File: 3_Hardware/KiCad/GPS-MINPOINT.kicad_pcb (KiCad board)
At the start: 2 copper layers, 2 parts, among them J1 110990030, U2 PIC24FJ64GA002-I/SP

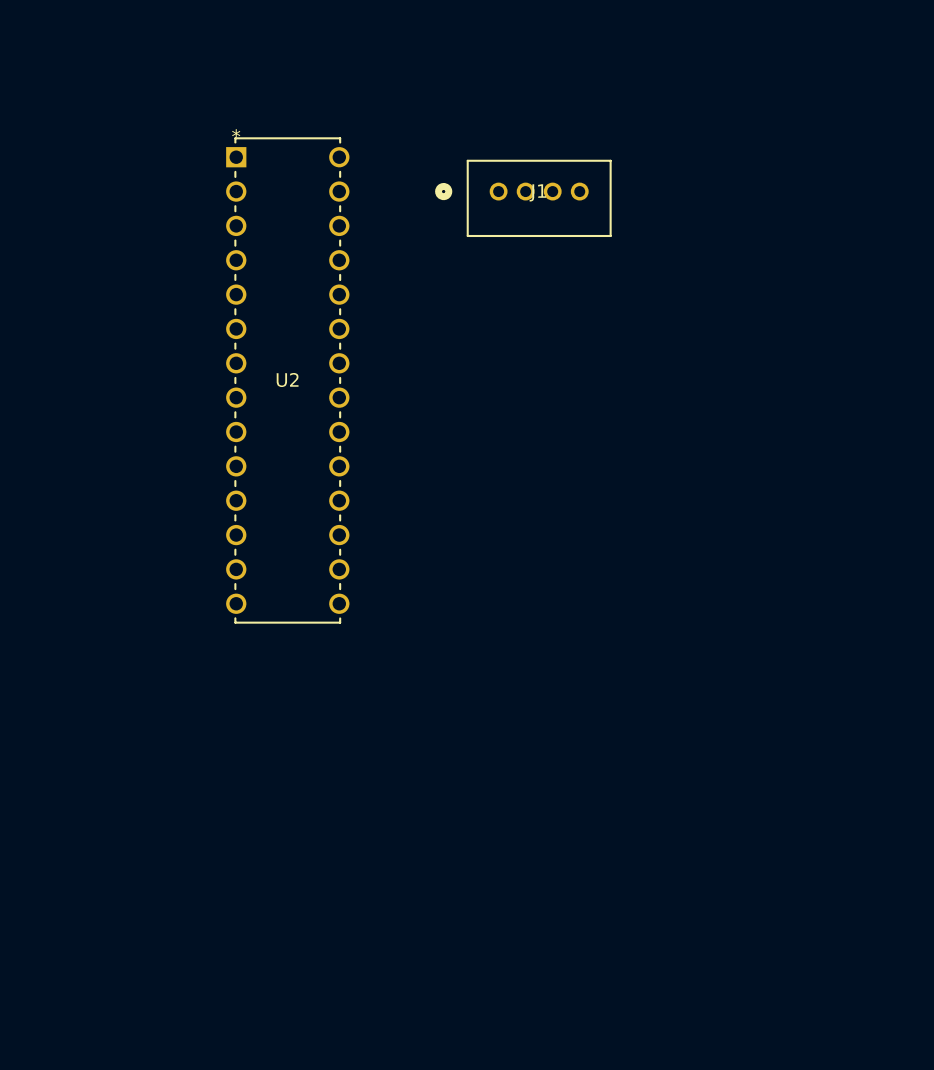
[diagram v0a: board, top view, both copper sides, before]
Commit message: Upload of finished PCB design
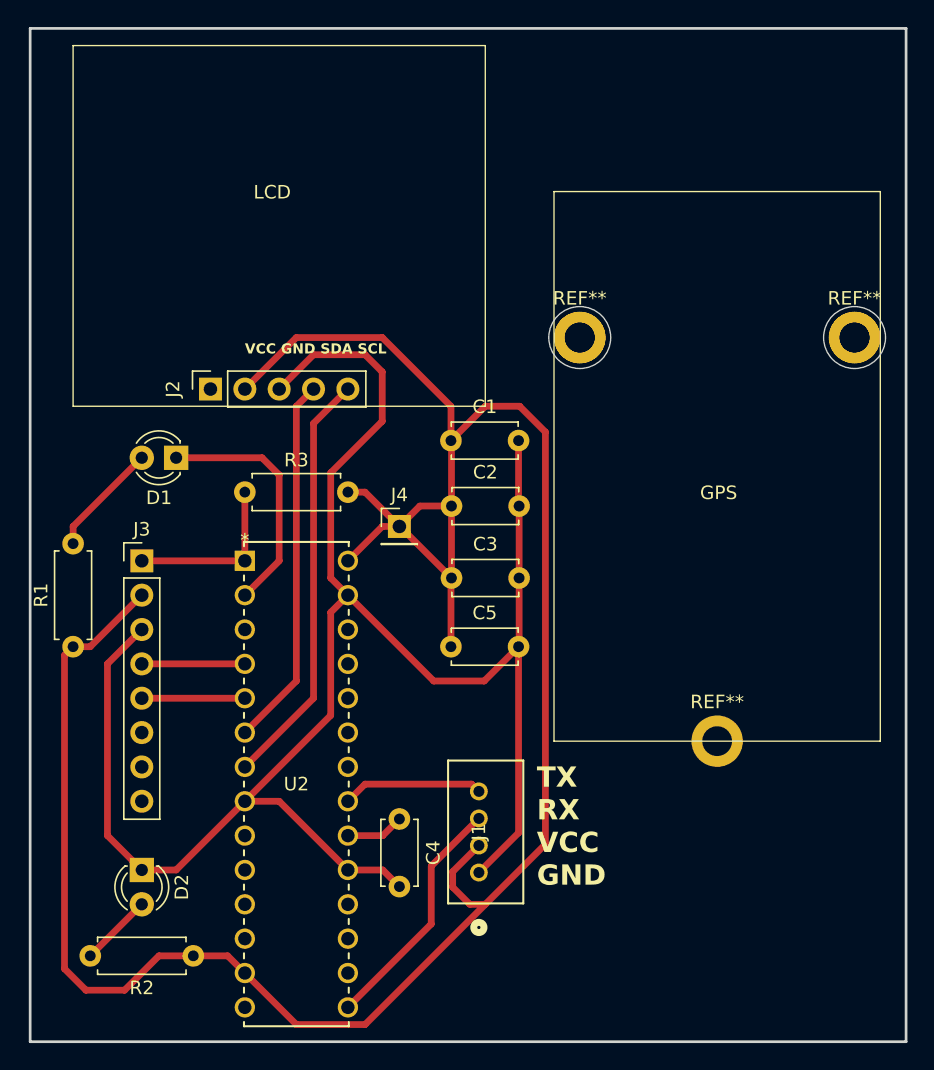
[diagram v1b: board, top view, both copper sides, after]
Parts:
- added ?: , , F.Cu at (167.6, 81.9)
- added ?: , , F.Cu at (188.0, 81.9)
- added C1: 10uF, Capacitor_THT:C_Disc_D4.7mm_W2.5mm_P5.00mm, F.Cu at (158.1, 89.5)
- added C2: 100nF, Capacitor_THT:C_Disc_D4.7mm_W2.5mm_P5.00mm, F.Cu at (158.2, 94.4)
- added C3: 100nF, Capacitor_THT:C_Disc_D4.7mm_W2.5mm_P5.00mm, F.Cu at (158.2, 99.7)
- added C4: 10uF, Capacitor_THT:C_Disc_D4.7mm_W2.5mm_P5.00mm, F.Cu at (154.3, 117.5)
- added C5: 10uF, Capacitor_THT:C_Disc_D4.7mm_W2.5mm_P5.00mm, F.Cu at (158.1, 104.8)
- added D1: G_LED, LED_THT:LED_D3.0mm, F.Cu at (137.8, 90.8)
- added D2: R_LED, LED_THT:LED_D3.0mm, F.Cu at (135.3, 121.3)
- added J2: LCD, Connector_PinSocket_2.54mm:PinSocket_1x05_P2.54mm_Vertical, F.Cu at (140.3, 85.7)
- added J3: ProgrammerConnector, Connector_PinHeader_2.54mm:PinHeader_1x08_P2.54mm_Vertical, F.Cu at (135.3, 98.4)
- added J4: PWR, Connector_PinHeader_2.54mm:PinHeader_1x01_P2.54mm_Vertical, F.Cu at (154.3, 95.9)
- added R1: 220, Resistor_THT:R_Axial_DIN0207_L6.3mm_D2.5mm_P7.62mm_Horizontal, F.Cu at (130.2, 104.8)
- added R2: 220, Resistor_THT:R_Axial_DIN0207_L6.3mm_D2.5mm_P7.62mm_Horizontal, F.Cu at (139.1, 127.6)
- added R3: 10k, Resistor_THT:R_Axial_DIN0207_L6.3mm_D2.5mm_P7.62mm_Horizontal, F.Cu at (142.9, 93.3)
- added REF**: MountingHole_2.2mm_M2_DIN965_Pad, MountingHole:MountingHole_2.2mm_M2_DIN965_Pad, F.Cu at (167.6, 81.9)
- added REF**: MountingHole_2.2mm_M2_DIN965_Pad, MountingHole:MountingHole_2.2mm_M2_DIN965_Pad, F.Cu at (188.0, 81.9)
- added REF**: MountingHole_2.2mm_M2_DIN965_Pad, MountingHole:MountingHole_2.2mm_M2_DIN965_Pad, F.Cu at (177.8, 111.8)
- moved J1 50.4 mm to (160.2, 121.5), turned to 90 degrees
- moved U2 29.9 mm to (142.9, 98.4)
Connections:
- J1 pad 1: Net-(J1-Pad1) -> Net-(D2-K)
- J1 pad 2: Net-(J1-Pad2) -> Net-(J1-VCC)
- J1 pad 3: unconnected-(J1-Pad3) -> Net-(J1-RX)
- J1 pad 4: unconnected-(J1-Pad4) -> Net-(J1-TX)
- U2 pad 1: unconnected-(U2-Pad1) -> Net-(J3-Pin_1)
- U2 pad 13: Net-(J1-Pad1) -> Net-(J1-VCC)
- U2 pad 15: unconnected-(U2-Pad15) -> Net-(J1-RX)
- U2 pad 19: unconnected-(U2-Pad19) -> Net-(D2-K)
- U2 pad 2: unconnected-(U2-Pad2) -> Net-(D1-K)
- U2 pad 20: unconnected-(U2-Pad20) -> Net-(C4-Pad1)
- U2 pad 21: unconnected-(U2-Pad21) -> Net-(J1-TX)
- U2 pad 27: Net-(J1-Pad2) -> Net-(D2-K)
- U2 pad 28: Net-(J1-Pad1) -> Net-(J1-VCC)
- U2 pad 4: unconnected-(U2-Pad4) -> Net-(J3-Pin_4)
- U2 pad 5: unconnected-(U2-Pad5) -> Net-(J3-Pin_5)
- U2 pad 6: unconnected-(U2-Pad6) -> Net-(J2-SDA)
- U2 pad 7: unconnected-(U2-Pad7) -> Net-(J2-SCL)
- U2 pad 8: Net-(J1-Pad2) -> Net-(D2-K)
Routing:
- net Net-(J1-VCC): track 0.00 -> 178.1 mm
- net Net-(D2-K): track 0.00 -> 139.4 mm
- net Net-(J2-SCL): track 0.00 -> 31.1 mm
- net Net-(J2-SDA): track 0.00 -> 27.5 mm
- net Net-(D1-K): track 0.00 -> 18.1 mm
- net Net-(J1-RX): track 0.00 -> 18.0 mm
- net Net-(J3-Pin_1): track 0.00 -> 12.7 mm
- net Net-(J1-TX): track 0.00 -> 10.4 mm
- net Net-(D1-A): track 0.00 -> 8.45 mm
- net Net-(J3-Pin_5): track 0.00 -> 7.62 mm
- net Net-(J3-Pin_4): track 0.00 -> 7.62 mm
- net Net-(D2-A): track 0.00 -> 5.39 mm
- net Net-(C4-Pad1): track 0.00 -> 4.32 mm
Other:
- board outline added: 64.8 x 74.9 mm
- board text added: "GPS"
- board text added: "LCD"
- board text added: "TX RX VCC GND"
- board text added: "VCC GND SDA SCL"
